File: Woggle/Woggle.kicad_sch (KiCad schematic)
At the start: 22 parts, among them J1 ICSP, SW1 SW_SPDT, SW2 SW_Push, U1 ATtiny85-20P

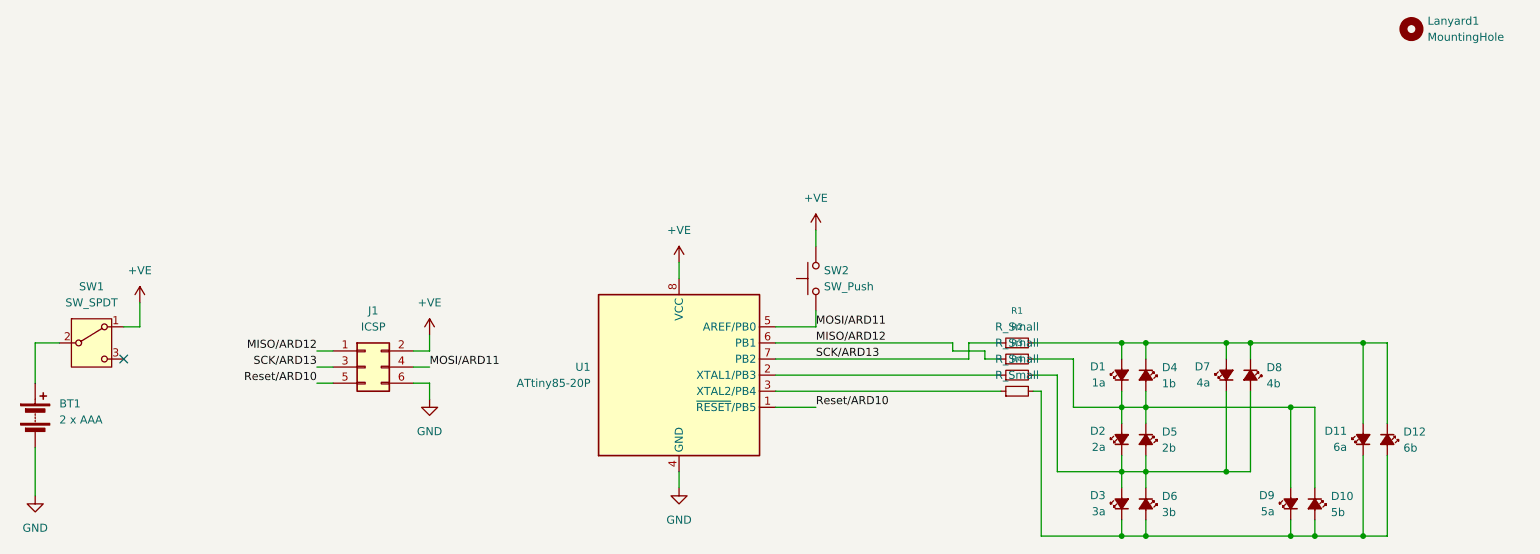
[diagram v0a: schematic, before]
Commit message: .
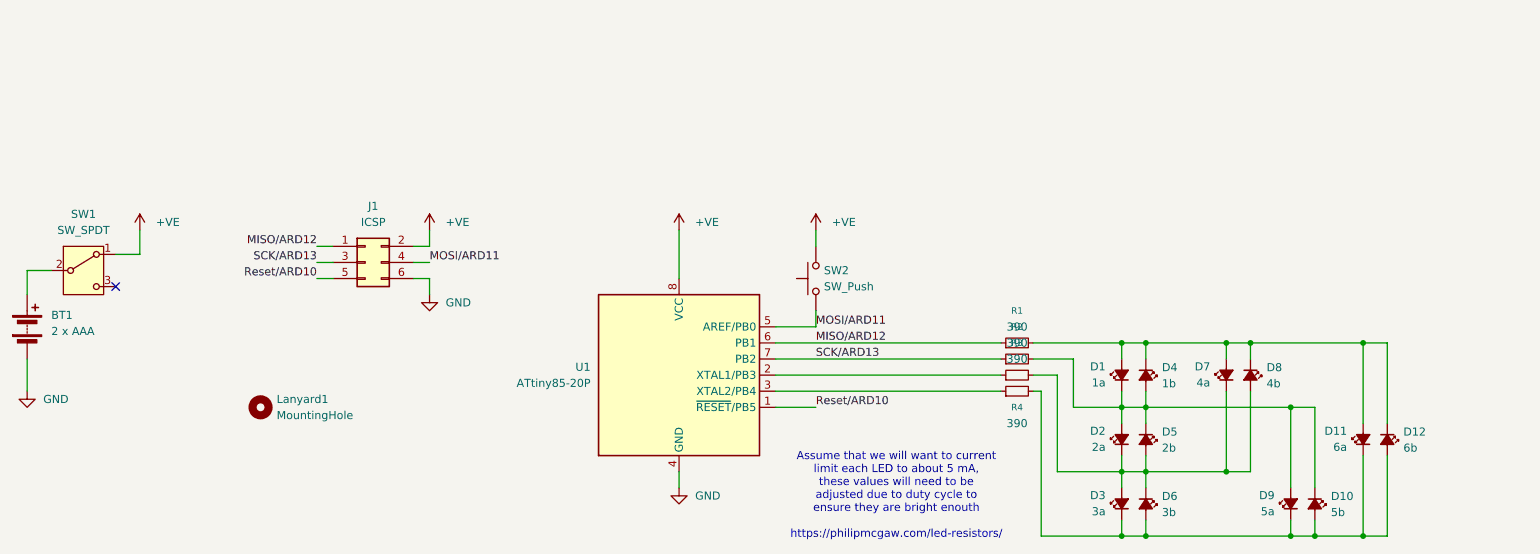
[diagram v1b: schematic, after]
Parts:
- J1: footprint Connector_PinHeader_2.54mm:PinHeader_2x03_P2.54mm_Vertical -> Connector:Tag-Connect_TC2030-IDC-NL_2x03_P1.27mm_Vertical
- R1, R2, R3, R4: value R_Small -> 390
- SW1: footprint (none) -> Button_Switch_THT:SW_Slide_SPDT_Angled_CK_OS102011MA1Q
- SW2: footprint (none) -> Button_Switch_THT:SW_PUSH-12mm
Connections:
- net MISO/ARD12: now also R1.1; no longer R2.1
- net SCK/ARD13: now also R2.1; no longer R1.1
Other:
- note added: "Assume that we will want to current limit each LED to about 5 mA, these values will need to be adjusted due to duty cycle to ensure they are bright enouth https://philipmcgaw.com/led-resistors/"
- moved on the sheet: BT1, J1, Lanyard1, SW1
